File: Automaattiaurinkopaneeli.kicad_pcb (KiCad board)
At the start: 2 copper layers, 39 parts, among them J1 Conn_02x04_Odd_Even, J10 Conn_01x16_Socket, J12 Conn_01x03_Socket, J13 Conn_01x05_Socket, J2 Conn_02x01, J3 Conn_01x02_Pin, J4 Conn_01x03_Pin, J5 Conn_01x03_Pin, J6 Conn_01x05_Pin, J7 Barrel_Jack_Switch, J8 Conn_01x02_Pin, J9 Conn_01x08_Socket, U1 ESP32-WROOM-32D, U2 ACS712xLCTR-20A, U3 LF33_TO220

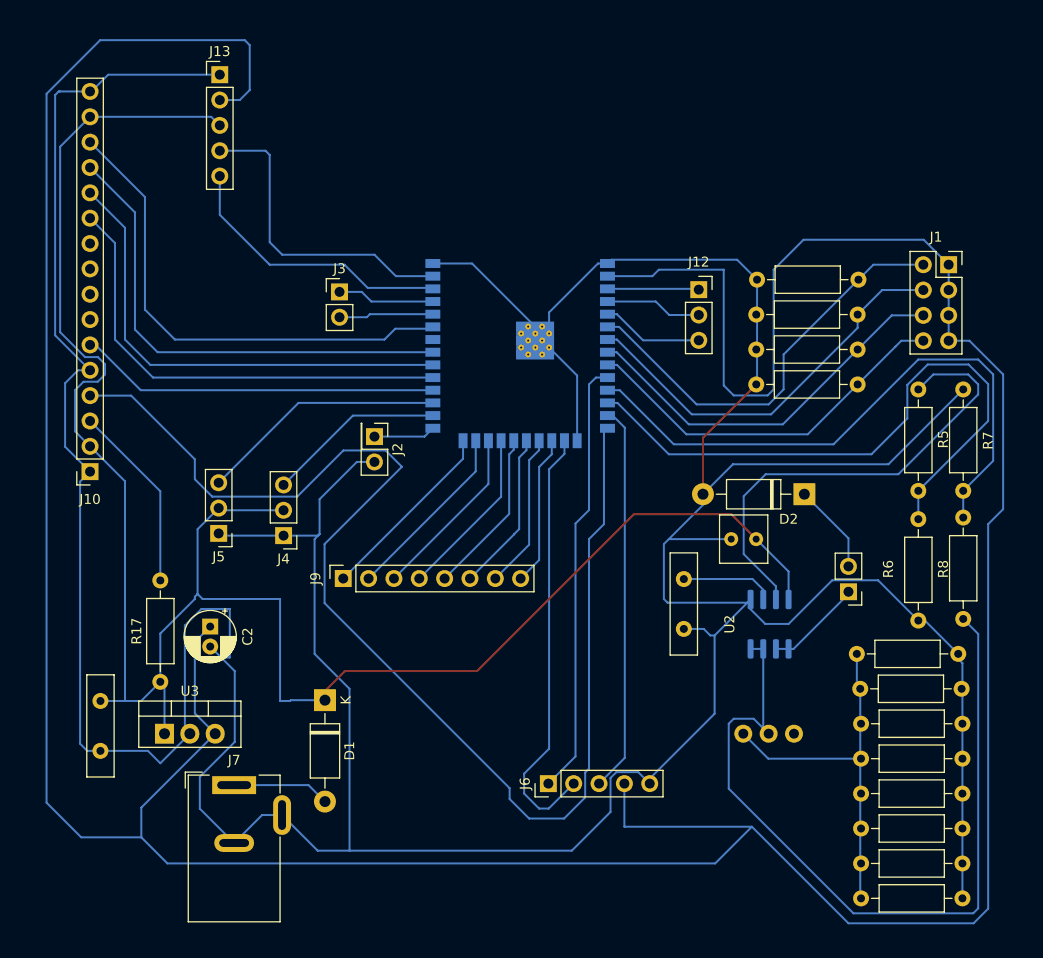
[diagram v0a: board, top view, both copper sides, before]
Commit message: V0.6
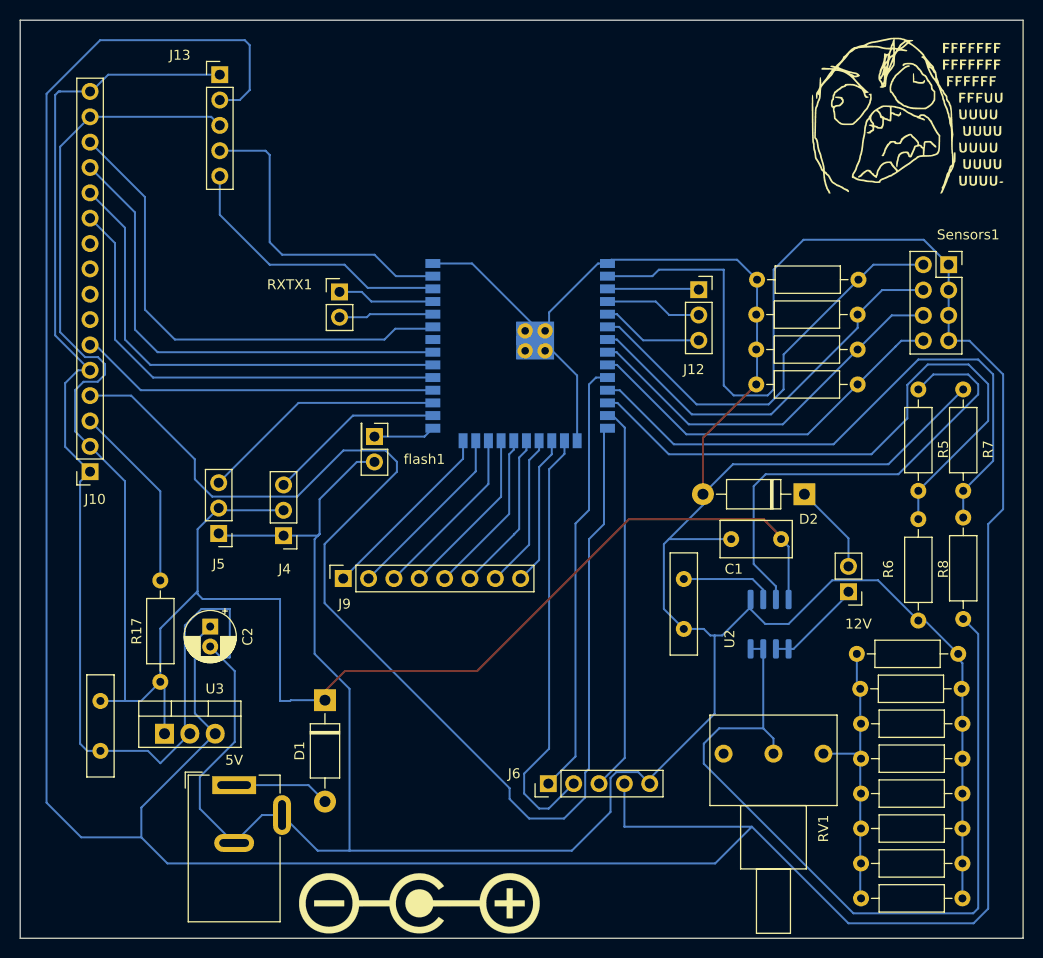
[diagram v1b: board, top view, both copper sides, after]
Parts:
- added G***: LOGO, generic:fuuuuuuuuuuuuuuuuuuuuuuuuuuuuuuuuuuuuuuuuuuuuuuuuuuuuuuuuuuuuuuuuuuuuuuuuuuuuuuuuuuuuuuuuuuuuu, F.Cu at (195.5, 30.5)
- added REF**: Polarity_Center_Positive_6mm_SilkScreen, Symbol:Polarity_Center_Positive_6mm_SilkScreen, F.Cu at (147.0, 109.5)
- C1: footprint Capacitor_THT:C_Rect_L4.6mm_W4.6mm_P2.50mm_MKS02_FKP02 -> Capacitor_THT:C_Rect_L7.0mm_W3.5mm_P5.00mm
- RV1: footprint Potentiometer_THT:Potentiometer_Vishay_148-149_Single_Horizontal -> generic:Potentiometer_Generic_148-149_Single_Horizontal; moved to F.Cu
- U1: footprint RF_Module:ESP32-WROOM-32D -> generic:ESP32-WROOM-32D
- moved RV1 2.87 mm to (182.5, 94.5)
- renumbered J8 to 12V, J7 to 5V, J3 to RXTX1, J1 to Sensors1, J2 to flash1
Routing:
- net Net-(R10-Pad2): track 37.5 -> 28.7 mm
- net Net-(D2-A): track 459.4 -> 454.7 mm
- net Net-(R8-Pad1): track 81.3 -> 84.3 mm
- net Net-(D1-K): track 202.5 -> 204.0 mm
- net Net-(U2-VIOUT): track 47.4 -> 46.6 mm
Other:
- board outline added: 100.5 x 92 mm
